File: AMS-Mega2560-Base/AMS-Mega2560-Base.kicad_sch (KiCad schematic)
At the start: 21 parts, among them J1 RTD1, J2 RTD2, J3 Conn_01x08, J4 Sense1, J5 Sense2, J6 AdafruitUltimateGPS, J7 Conn_02x03_Odd_Even, P1 Power, P10 CONN_01X01, P11 CONN_01X01, P12 CONN_01X01, P13 CONN_01X01, P2 Analog, P3 Analog, P4 Digital, P5 PWM, P6 PWM, P7 Communication, P8 CONN_01X01, P9 CONN_01X01

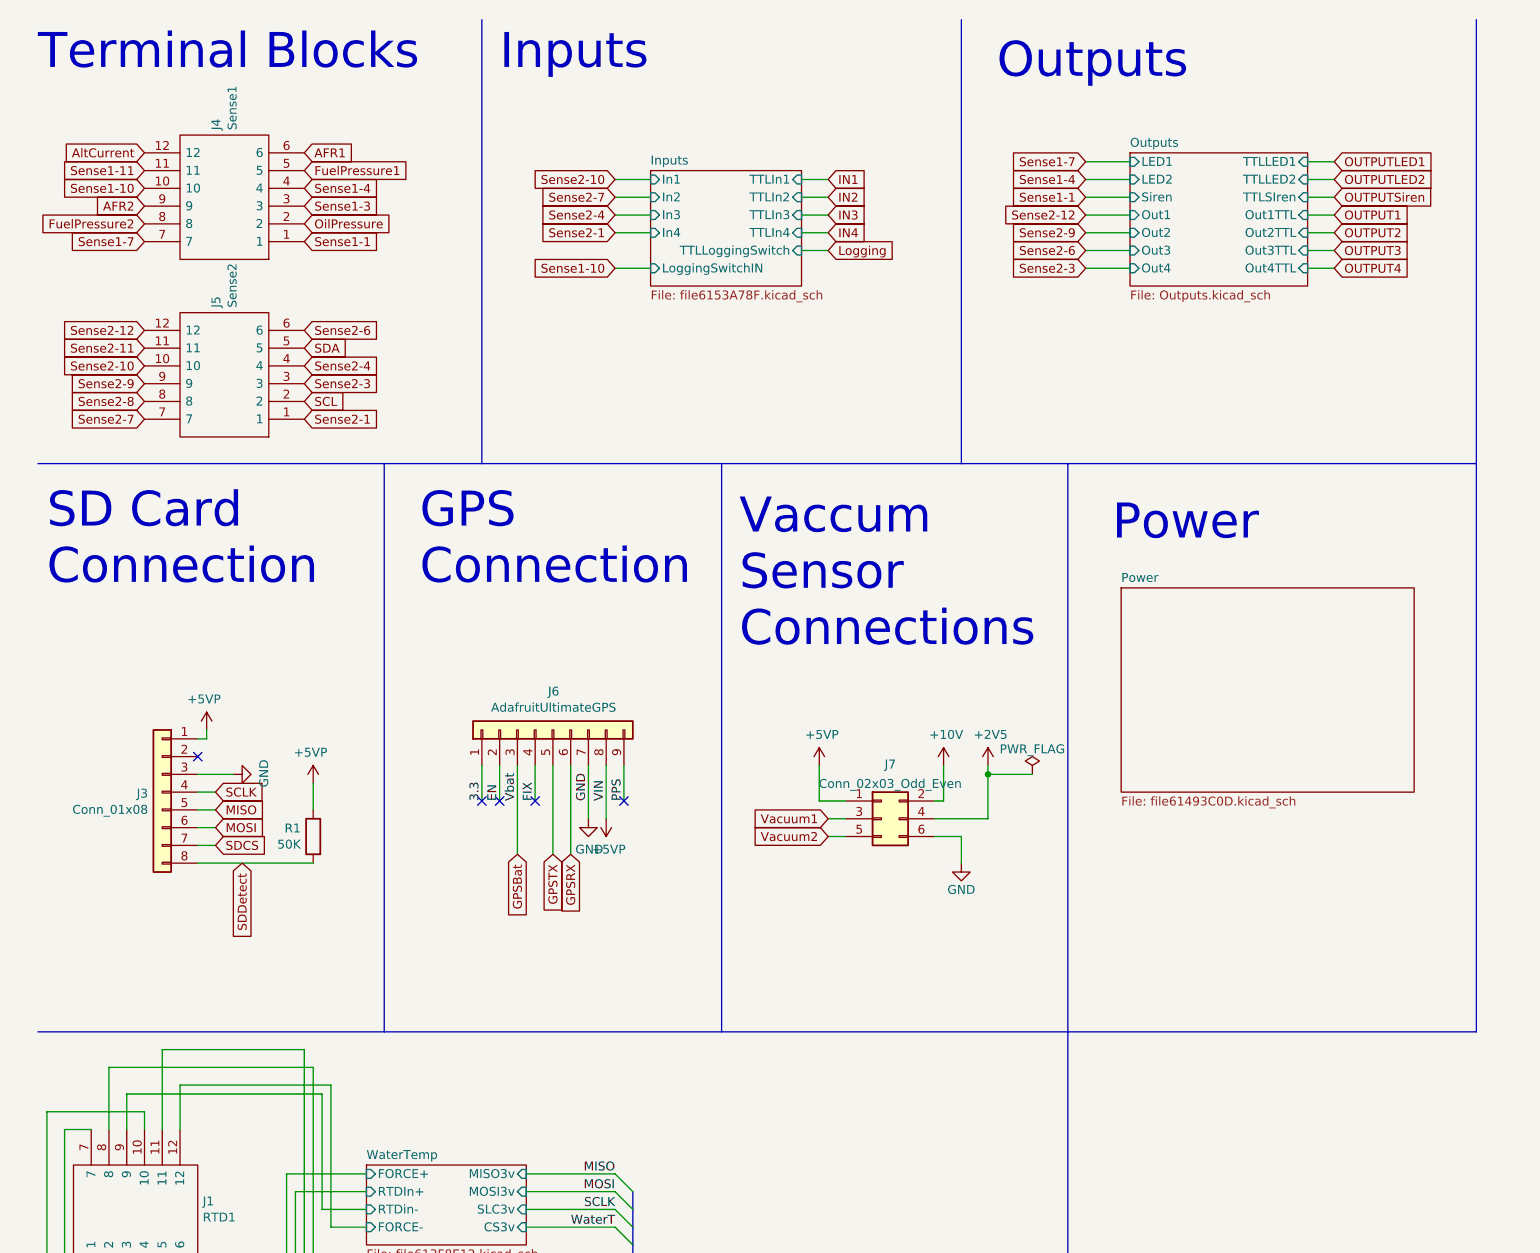
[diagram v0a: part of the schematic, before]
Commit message: wip for the base PCB, finished Vacuum PCB and Fab Files for that.
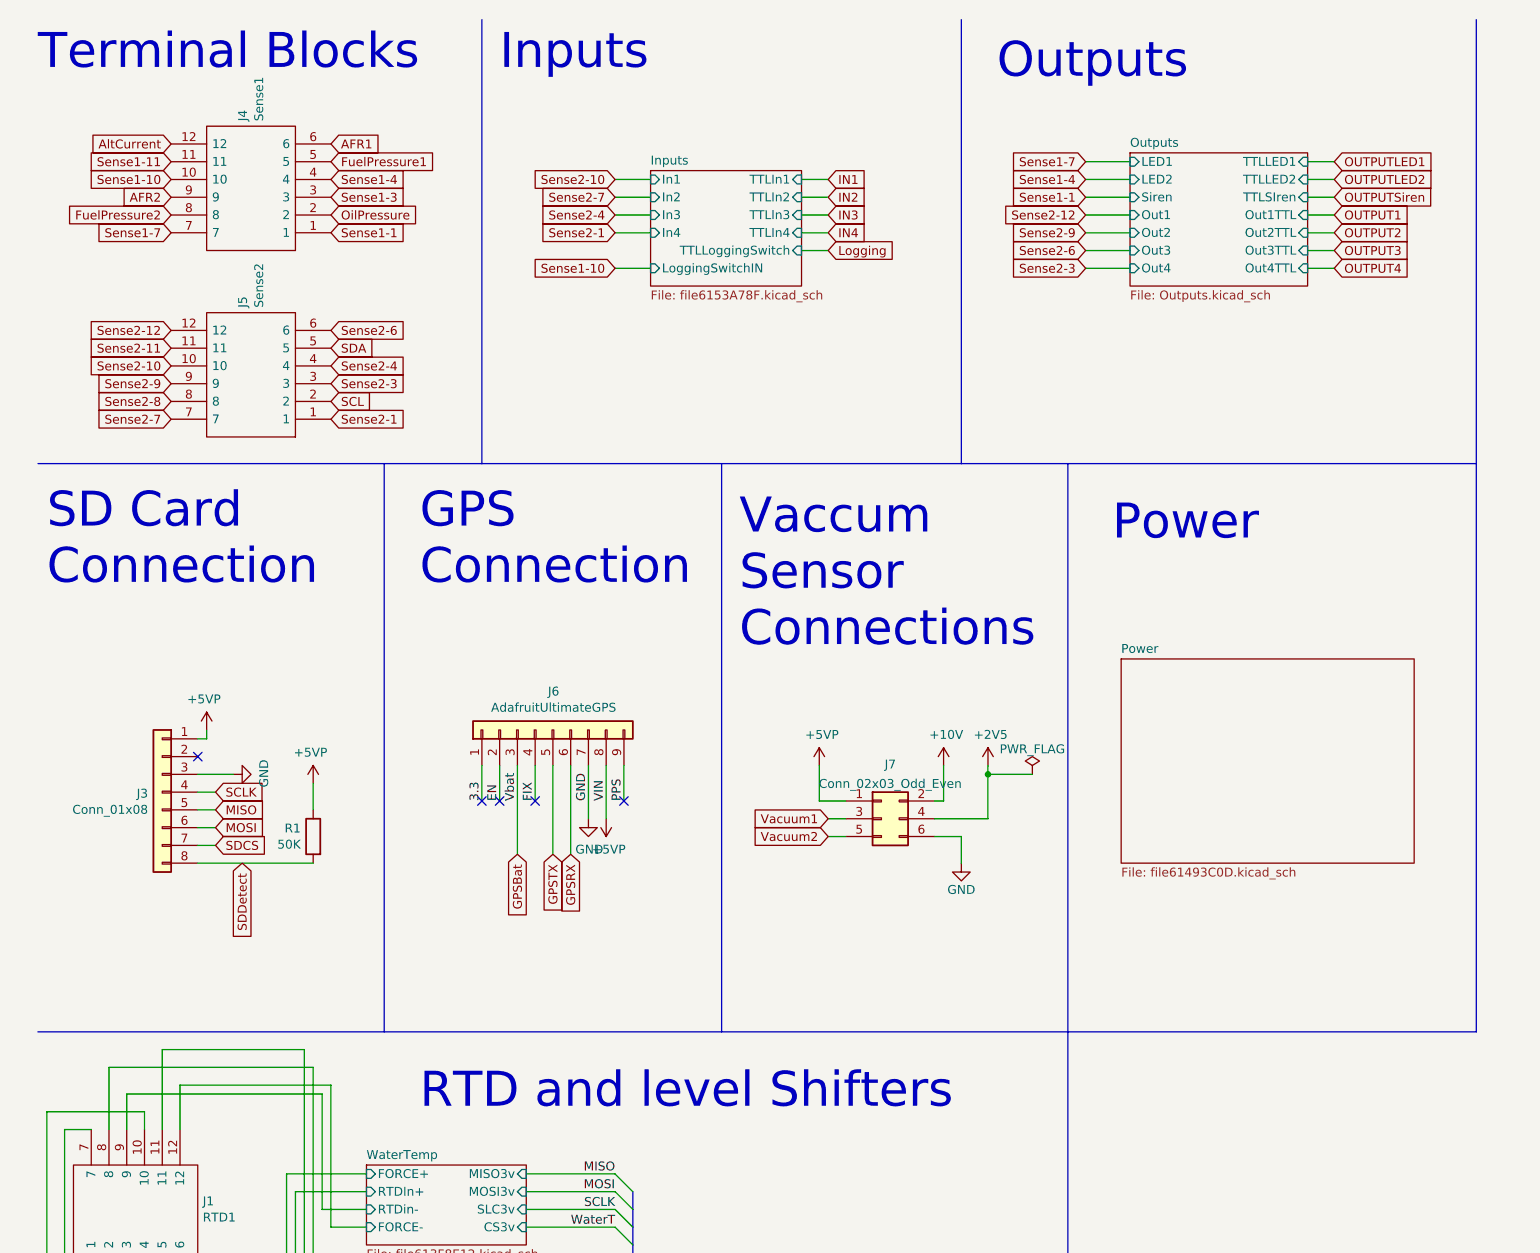
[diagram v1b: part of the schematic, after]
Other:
- note added: "RTD and level Shifters"
- moved on the sheet: J4, J5

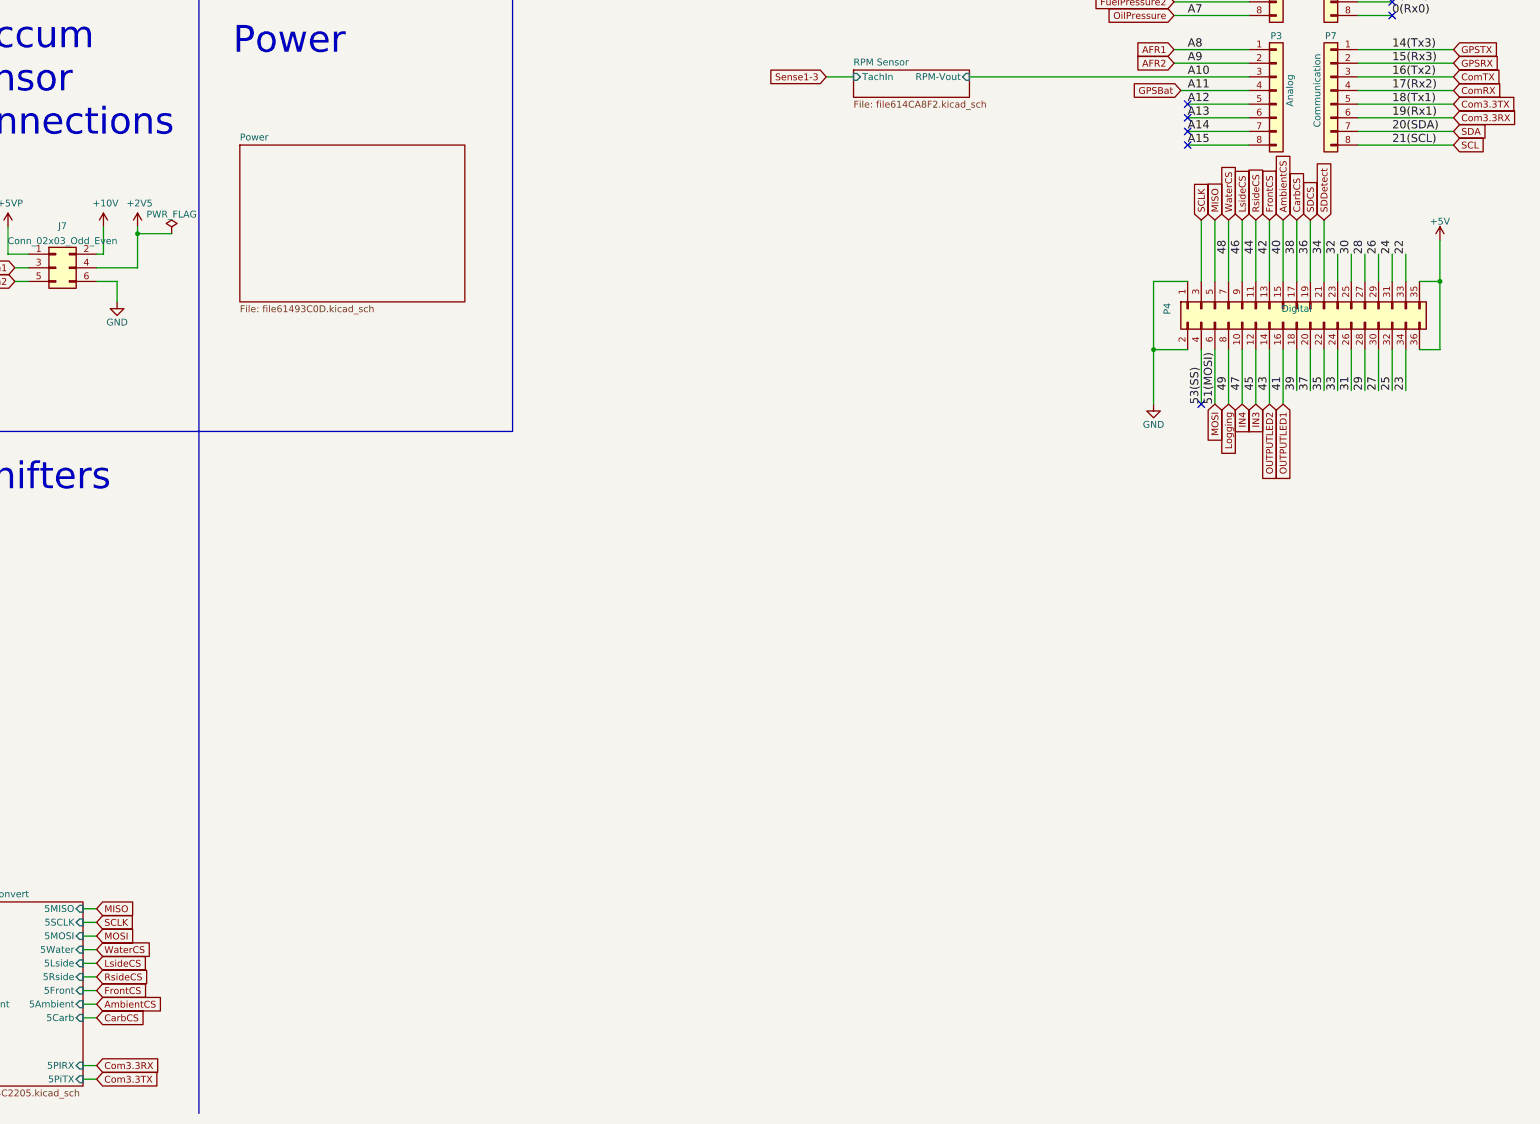
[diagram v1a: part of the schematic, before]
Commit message: WIP for layout
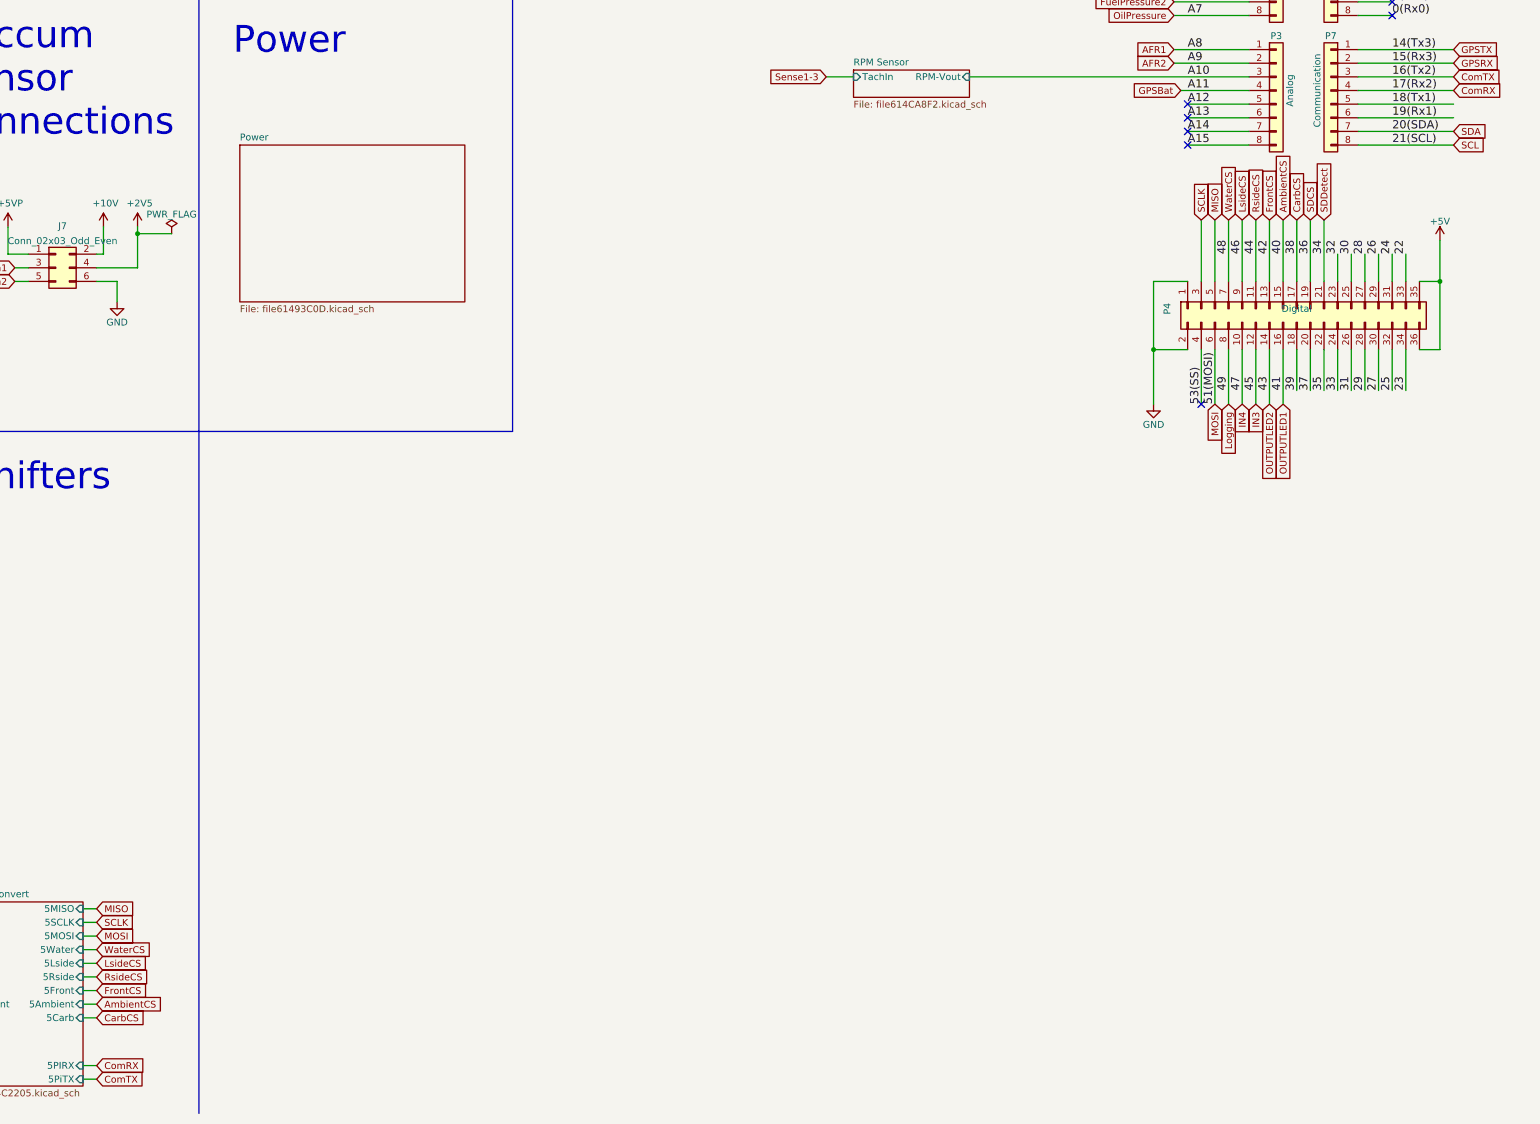
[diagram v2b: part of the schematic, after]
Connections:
- net Com3.3RX renamed 19(Rx1)
- net Com3.3TX renamed 18(Tx1)
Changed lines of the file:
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@@
+    )
+  )
+  (global_label "ComRX" (shape input) (at 140.97 275.59 0) (fields_autoplaced)
+    (effects (font (size 1.27 1.27)) (justify left))
+    (property "Intersheet References" "${INTERSHEET_REFS}" (id 0) (at -134.62 181.61 0)
+      (effects (font (size 1.27 1.27)) hide)
     )
   )
@@
     )
   )
-  (global_label "Com3.3TX" (shape input) (at 140.97 278.13 0) (fields_autoplaced)
-    (effects (font (size 1.27 1.27)) (justify left))
-    (property "Intersheet References" "${INTERSHEET_REFS}" (id 0) (at -5.08 83.82 0)
-      (effects (font (size 1.27 1.27)) hide)
-    )
-  )
   (global_label "FuelPressure1" (shape input) (at 341.63 74.93 180) (fields_autoplaced)
     (effects (font (size 1.27 1.27)) (justify right))
@@
     )
   )
-  (global_label "Com3.3RX" (shape input) (at 393.7 99.06 0) (fields_autoplaced)
-    (effects (font (size 1.27 1.27)) (justify left))
-    (property "Intersheet References" "${INTERSHEET_REFS}" (id 0) (at 118.11 0 0)
-      (effects (font (size 1.27 1.27)) hide)
-    )
-  )
   (global_label "IN4" (shape input) (at 354.33 152.4 270) (fields_autoplaced)
     (effects (font (size 1.27 1.27)) (justify right))
@@
     )
   )
-  (global_label "Com3.3TX" (shape input) (at 393.7 96.52 0) (fields_autoplaced)
-    (effects (font (size 1.27 1.27)) (justify left))
-    (property "Intersheet References" "${INTERSHEET_REFS}" (id 0) (at 118.11 0 0)
-      (effects (font (size 1.27 1.27)) hide)
-    )
-  )
   (global_label "ComTX" (shape input) (at 393.7 91.44 0) (fields_autoplaced)
     (effects (font (size 1.27 1.27)) (justify left))
@@
     )
   )
-  (global_label "Com3.3RX" (shape input) (at 140.97 275.59 0) (fields_autoplaced)
-    (effects (font (size 1.27 1.27)) (justify left))
-    (property "Intersheet References" "${INTERSHEET_REFS}" (id 0) (at -5.08 83.82 0)
-      (effects (font (size 1.27 1.27)) hide)
-    )
-  )
   (global_label "Sense2-12" (shape input) (at 31.75 57.15 180) (fields_autoplaced)
     (effects (font (size 1.27 1.27)) (justify right))
@@
     )
   )
+  (global_label "ComTX" (shape input) (at 140.97 278.13 0) (fields_autoplaced)
+    (effects (font (size 1.27 1.27)) (justify left))
+    (property "Intersheet References" "${INTERSHEET_REFS}" (id 0) (at -134.62 186.69 0)
+      (effects (font (size 1.27 1.27)) hide)
+    )
+  )
